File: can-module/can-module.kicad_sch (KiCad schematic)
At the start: 17 parts, among them IC1 PIC32CM1216JH01048-I_U5B

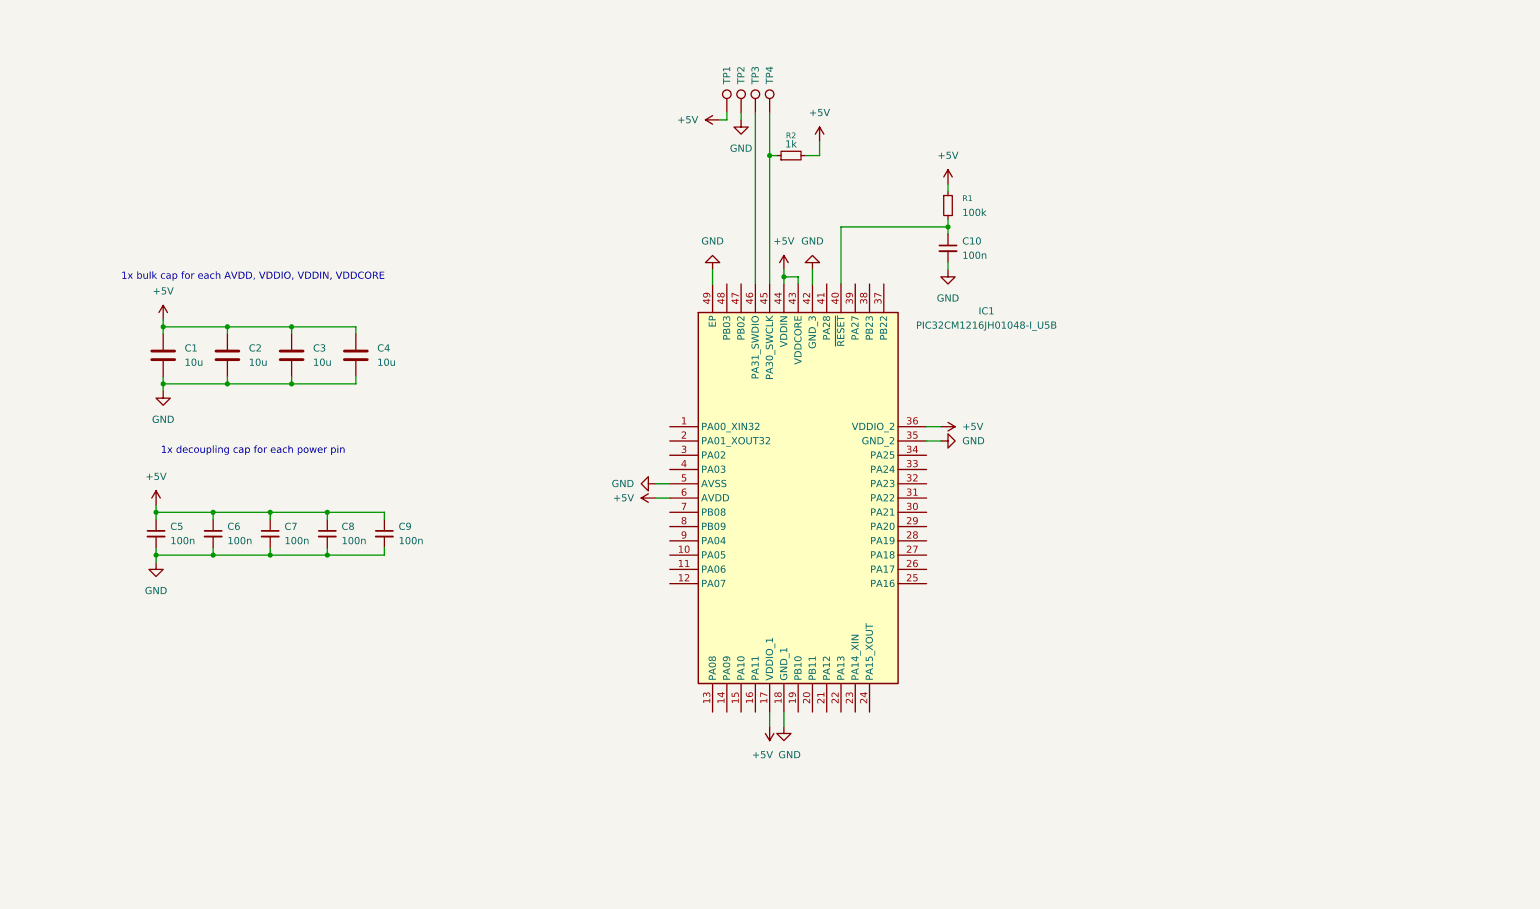
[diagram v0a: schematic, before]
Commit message: can-module: Add ATA6560 CAN transceiver
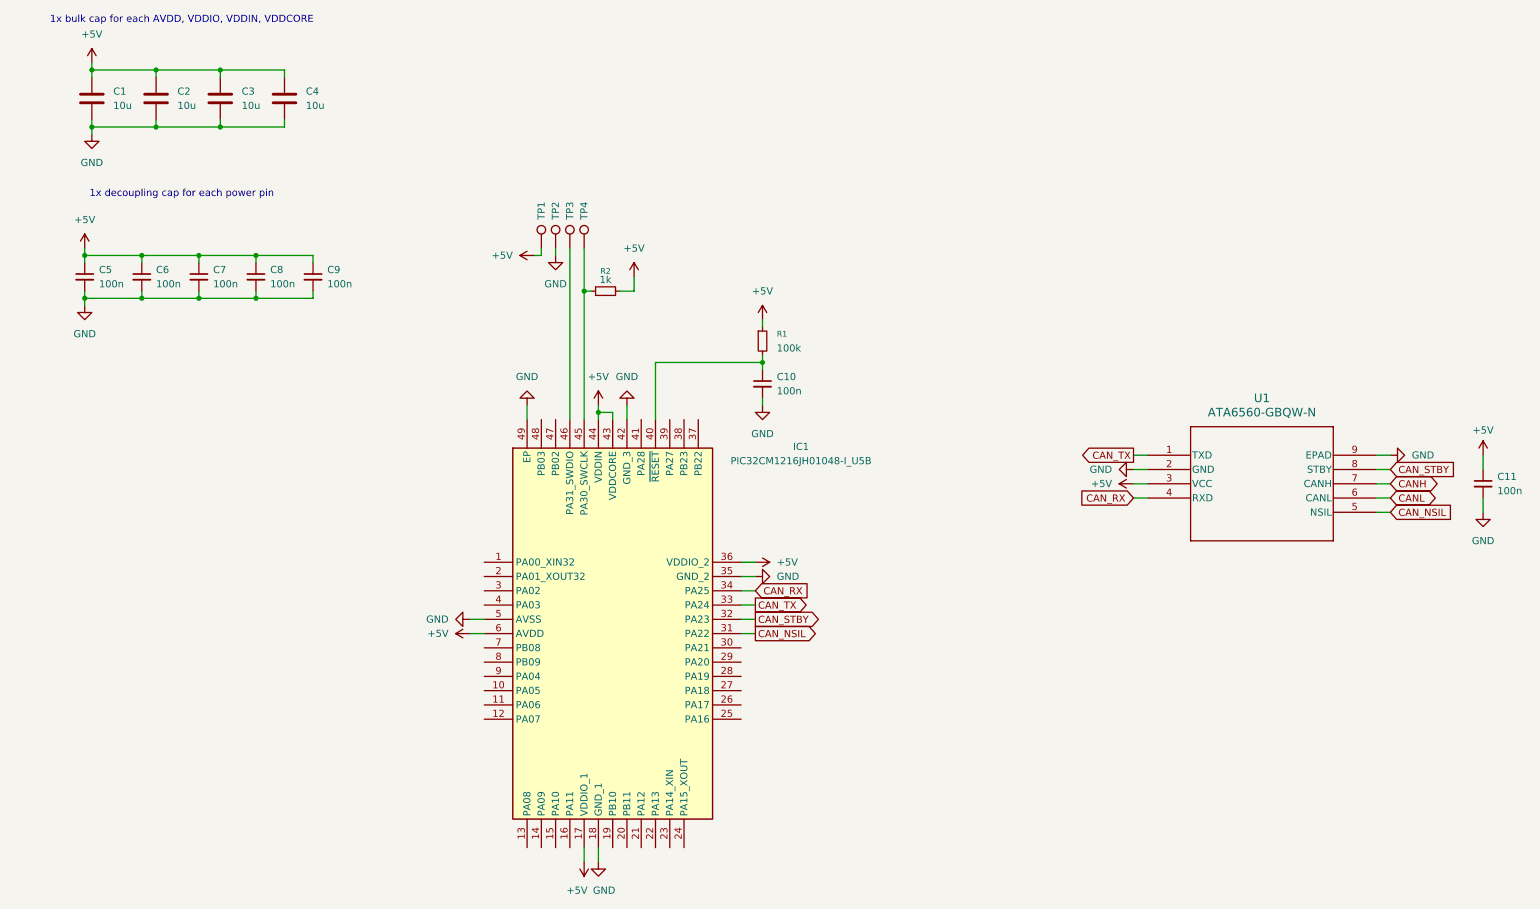
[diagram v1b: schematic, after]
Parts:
- added C11: 100n, Capacitor_SMD:C_0201_0603Metric, symbol Device:C_Small
- added U1: ATA6560-GBQW-N, VDFN8_3X3_MCH, symbol ATA6560-GBQW-N:ATA6560-GBQW-N
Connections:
- net +5V: now also C11.1, U1.3 (VCC)
- net GND: now also C11.2, U1.2 (GND), U1.9 (EPAD)
- net CAN_NSIL: now reaches IC1.31 (PA22)
- net CAN_NSIL: now also U1.5 (NSIL)
- net CAN_STBY: now reaches IC1.32 (PA23)
- net CAN_STBY: now also U1.8 (STBY)
- net CAN_TX: now reaches IC1.33 (PA24)
- net CAN_TX: now also U1.1 (TXD)
- net CAN_RX: now reaches IC1.34 (PA25)
- net CAN_RX: now also U1.4 (RXD)
- new net CANH: U1.7 (CANH)
- new net CANL: U1.6 (CANL)
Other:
- moved on the sheet: C1, C10, C2, C3, C4, C5, C6, C7, C8, C9, IC1, R1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
